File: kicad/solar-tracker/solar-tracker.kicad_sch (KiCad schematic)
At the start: 2 parts, among them J1 Barrel_Jack_Switch

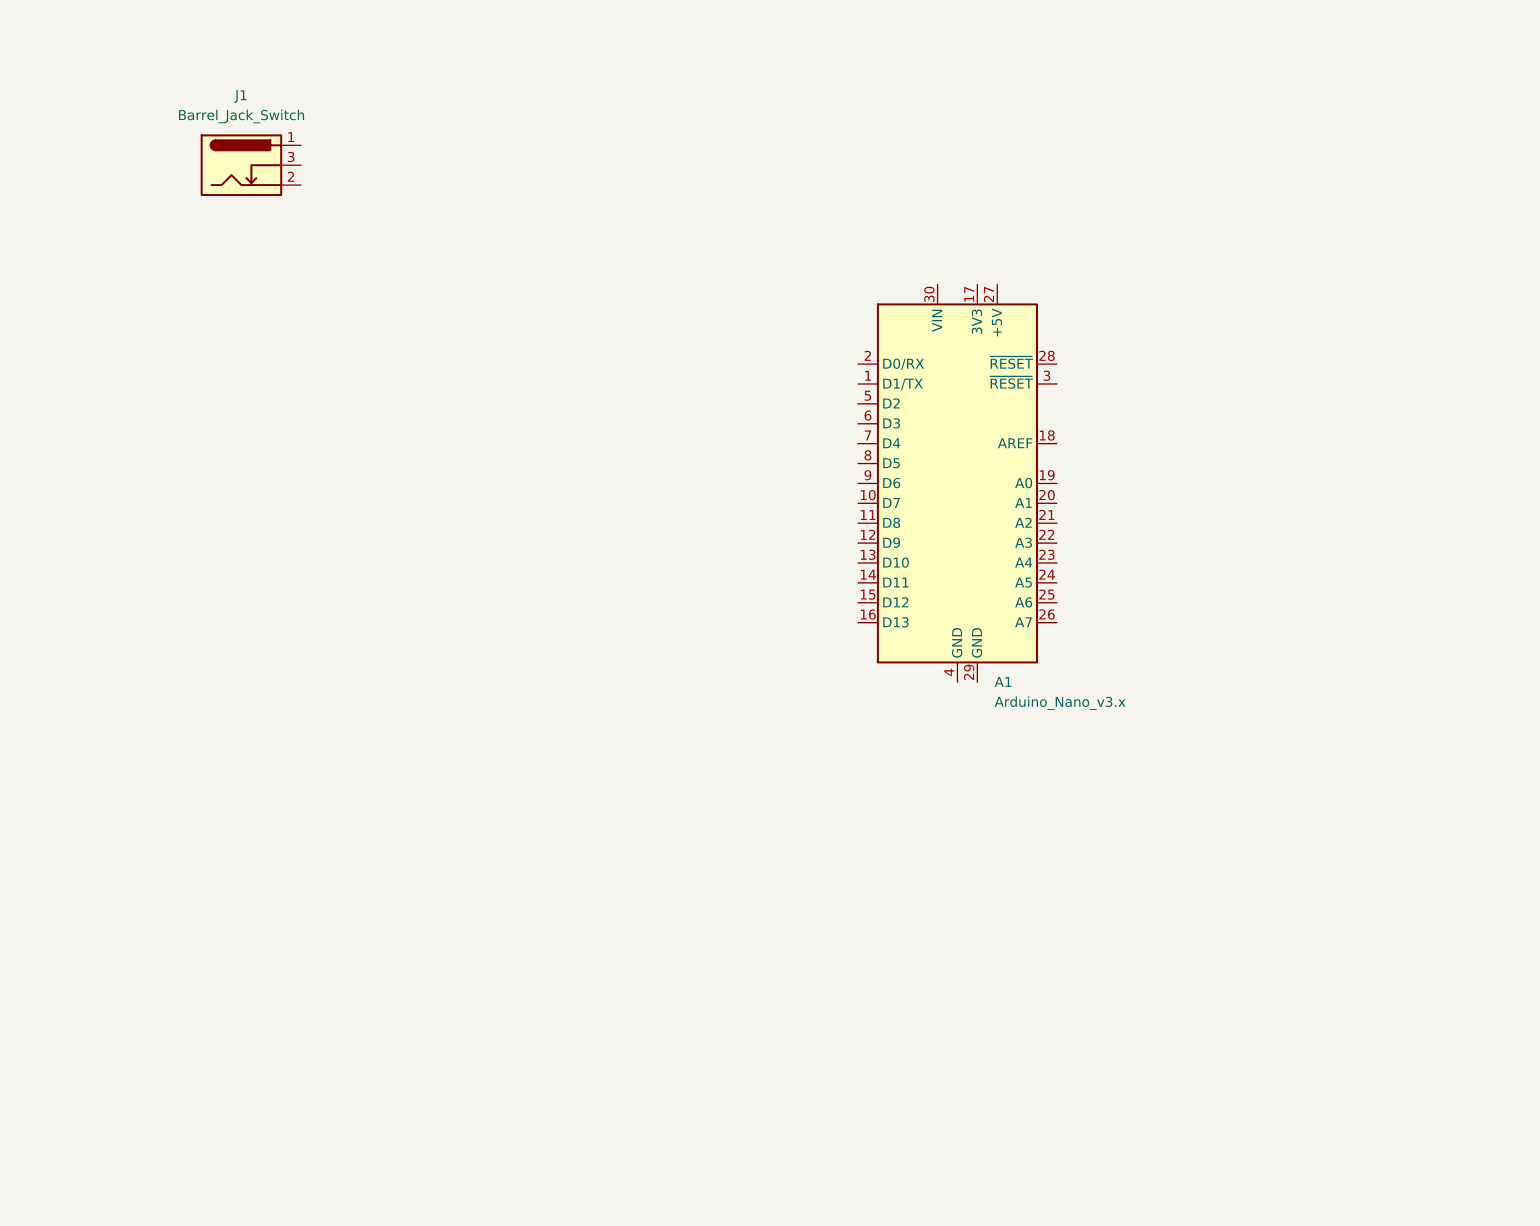
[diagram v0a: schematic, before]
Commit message: update
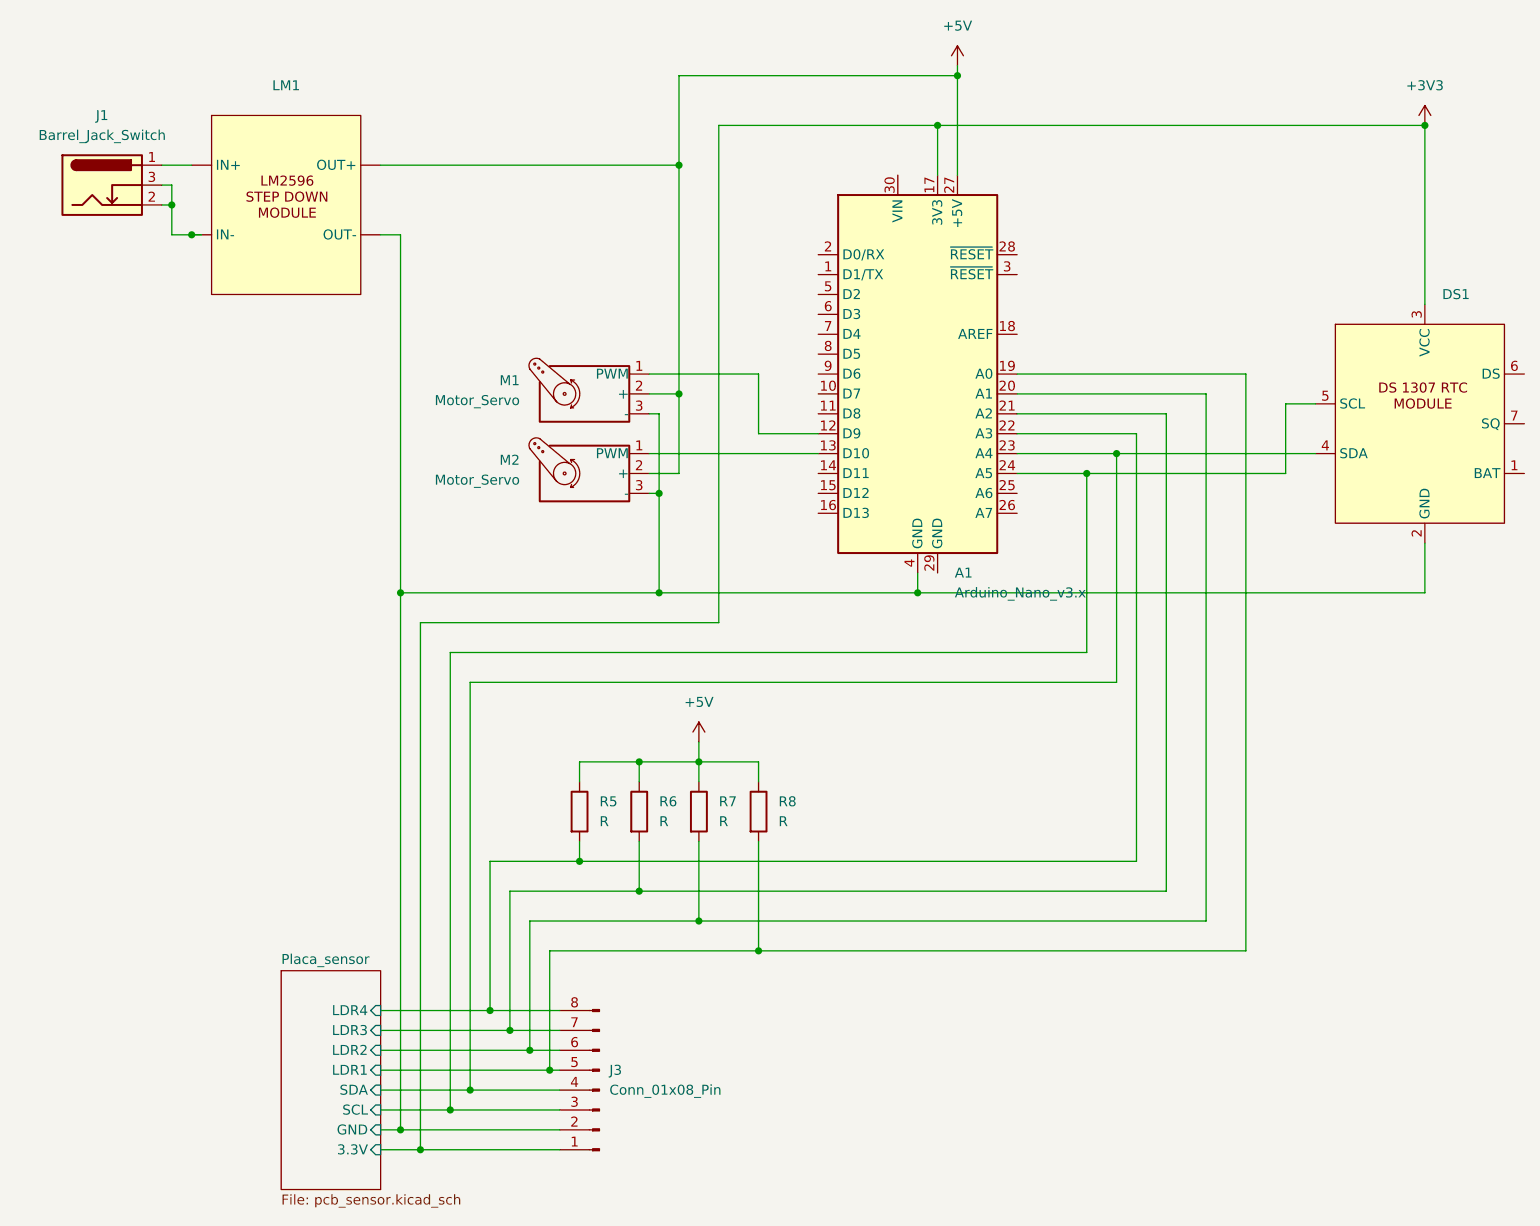
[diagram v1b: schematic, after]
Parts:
- added DS1: ~, arduino_modulos:DS1307_RTC_MODULE, symbol arduino_modulos:DS_1307_RTC_Module
- added J3: Conn_01x08_Pin, solar_tracker:PinHeader_1x08_P2.54mm_Vertical_large_pad, symbol solar_tracker:Conn_01x08_Pin
- added LM1: ~, arduino_modulos:LM2596_Step_Down_module, symbol arduino_modulos:LM_2596_Step_Down_Module
- added M1, M2: Motor_Servo, Connector_PinHeader_2.54mm:PinHeader_1x03_P2.54mm_Vertical, symbol Motor:Motor_Servo
- added R5, R6, R7, R8: R, solar_tracker:resistor_250mw_12mm, symbol Device:R
- J1: footprint (none) -> solar_tracker:BarrelJack_Horizontal
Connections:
- net at J1.1: now also LM1. (OUT-)
- net at J1.2: now also J1.3, LM1. (OUT-)
- net at A1.12 (D9): now also M1.1 (PWM)
- net at A1.13 (D10): now also M2.1 (PWM)
- net +3V3: now reaches A1.17 (3V3)
- net +3V3: now also DS1.3 (VCC), J3.1 (Pin_1)
- net Placa_sensor/LDR1: now reaches A1.19 (A0)
- net Placa_sensor/LDR1: now also J3.5 (Pin_5), R8.2
- net Placa_sensor/LDR2: now reaches A1.20 (A1)
- net Placa_sensor/LDR2: now also J3.6 (Pin_6), R7.2
- net Placa_sensor/LDR3: now reaches A1.21 (A2)
- net Placa_sensor/LDR3: now also J3.7 (Pin_7), R6.2
- net Placa_sensor/LDR4: now reaches A1.22 (A3)
- net Placa_sensor/LDR4: now also J3.8 (Pin_8), R5.2
- net Placa_sensor/SDA: now reaches A1.23 (A4)
- net Placa_sensor/SDA: now also DS1.4 (SDA), J3.4 (Pin_4)
- net Placa_sensor/SCL: now reaches A1.24 (A5)
- net Placa_sensor/SCL: now also DS1.5 (SCL), J3.3 (Pin_3)
- net +5V: now reaches A1.27 (+5V)
- net +5V: now also LM1. (OUT-), M1.2 (+), M2.2 (+), R5.1, R6.1, R7.1, R8.1
- net Placa_sensor/GND: now reaches A1.4 (GND)
- net Placa_sensor/GND: now also DS1.2 (GND), J3.2 (Pin_2), LM1. (OUT-), M1.3 (-), M2.3 (-)
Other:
- added sheet Placa_sensor (pcb_sensor.kicad_sch)
- moved on the sheet: A1, J1
